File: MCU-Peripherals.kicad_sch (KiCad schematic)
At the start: 2 parts, among them J1 Conn_01x05, SW1 SW_Push

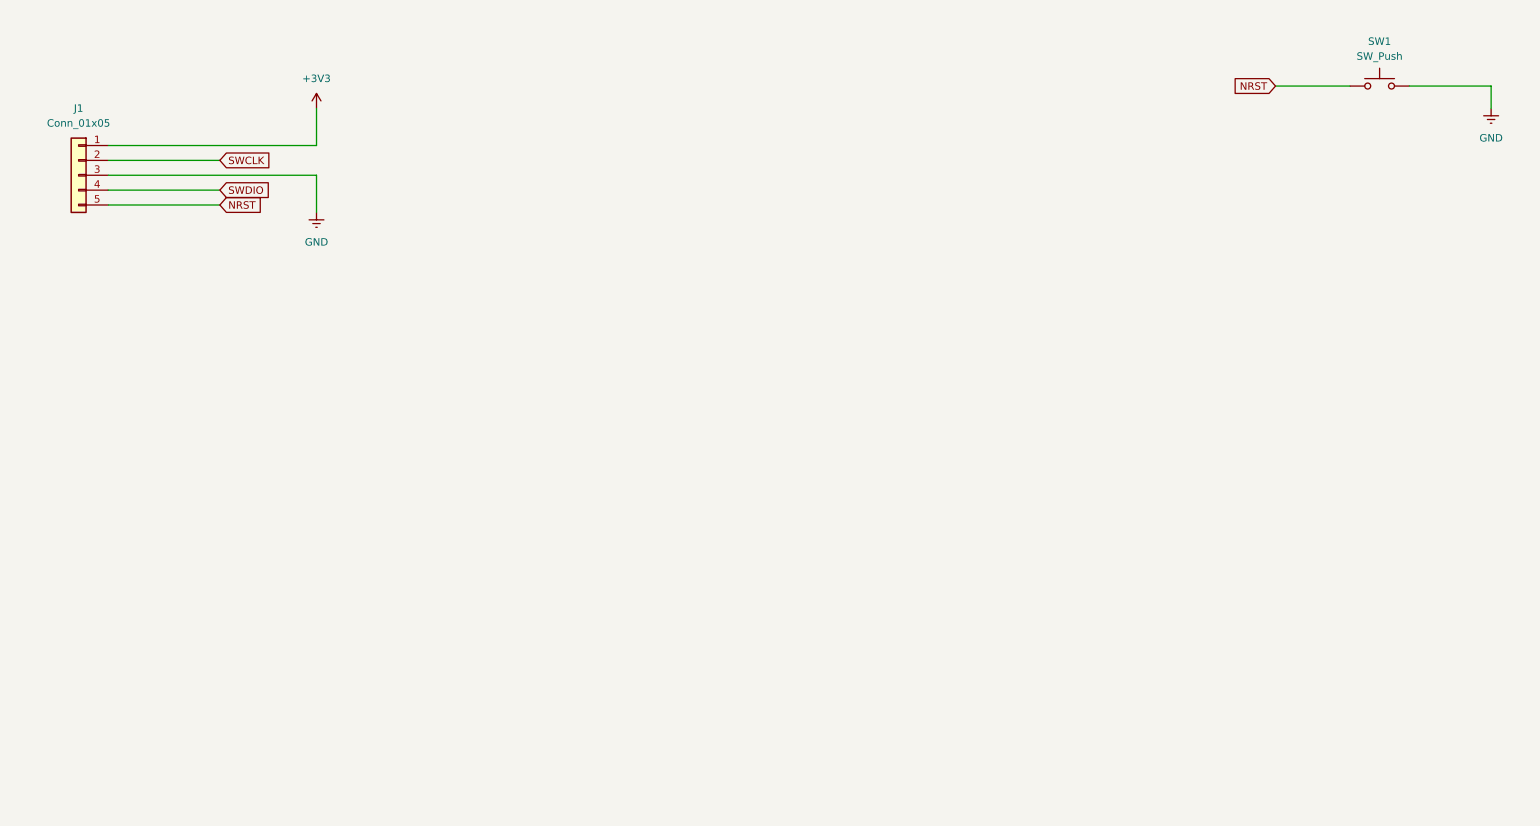
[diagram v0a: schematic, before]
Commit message: Decent progress, started USB
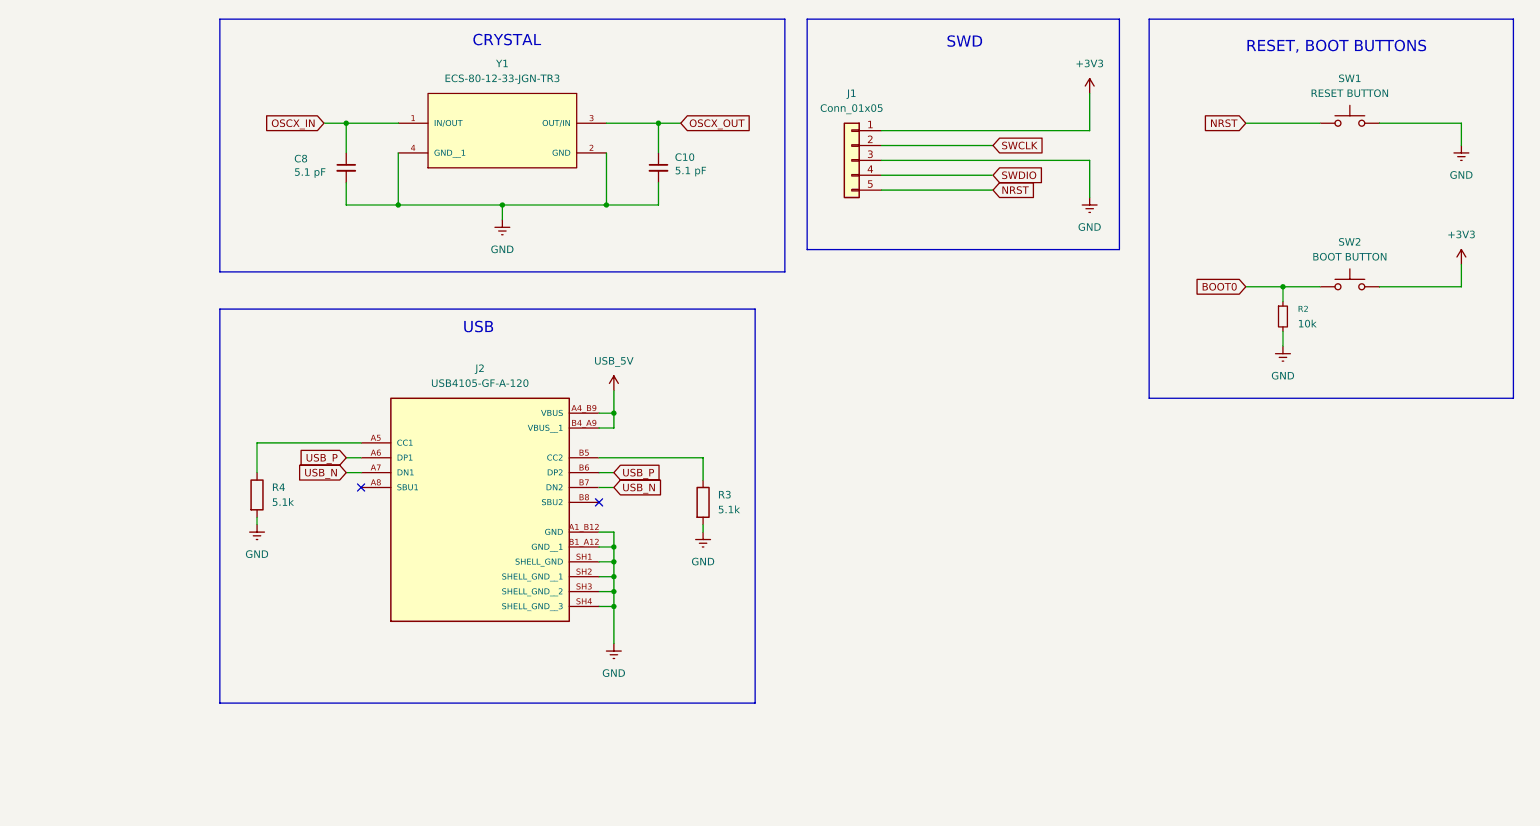
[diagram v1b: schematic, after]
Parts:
- added C10, C8: 5.1 pF, symbol Device:C_Small
- added J2: USB4105-GF-A-120, USB4105-GF-A-120:GCT_USB4105-GF-A-120, symbol USB4105-GF-A-120:USB4105-GF-A-120
- added R2: 10k, symbol Device:R_Small
- added R3, R4: 5.1k, symbol Device:R
- added SW2: BOOT BUTTON, symbol Switch:SW_Push
- added Y1: ECS-80-12-33-JGN-TR3, ECS-80-12-33-JGN-TR3:XTAL_ECS-240-8-33-AGN-TR, symbol ECS-80-12-33-JGN-TR3:ECS-80-12-33-JGN-TR3
- SW1: value SW_Push -> RESET BUTTON
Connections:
- net +3V3: now also SW2.2
- net GND: now also C10.2, C8.2, J2.A1_B12 (GND), J2.B1_A12 (GND__1), J2.SH1 (SHELL_GND), J2.SH2 (SHELL_GND__1), J2.SH3 (SHELL_GND__2), J2.SH4 (SHELL_GND__3), R2.2, R3.2, R4.2, Y1.2 (GND), Y1.4 (GND__1)
- new net: J2.A5 (CC1), R4.1
- new net: J2.B5 (CC2), R3.1
- new net BOOT0: R2.1, SW2.1
- new net OSCX_IN: C8.1, Y1.1 (IN/OUT)
- new net OSCX_OUT: C10.1, Y1.3 (OUT/IN)
- new net USB_5V: J2.A4_B9 (VBUS), J2.B4_A9 (VBUS__1)
- new net USB_N: J2.A7 (DN1), J2.B7 (DN2)
- new net USB_P: J2.A6 (DP1), J2.B6 (DP2)
- no-connect marks 0 -> 2
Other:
- note added: "CRYSTAL"
- note added: "RESET, BOOT BUTTONS"
- note added: "SWD"
- note added: "USB"
- moved on the sheet: J1, SW1

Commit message: Further schematic progress
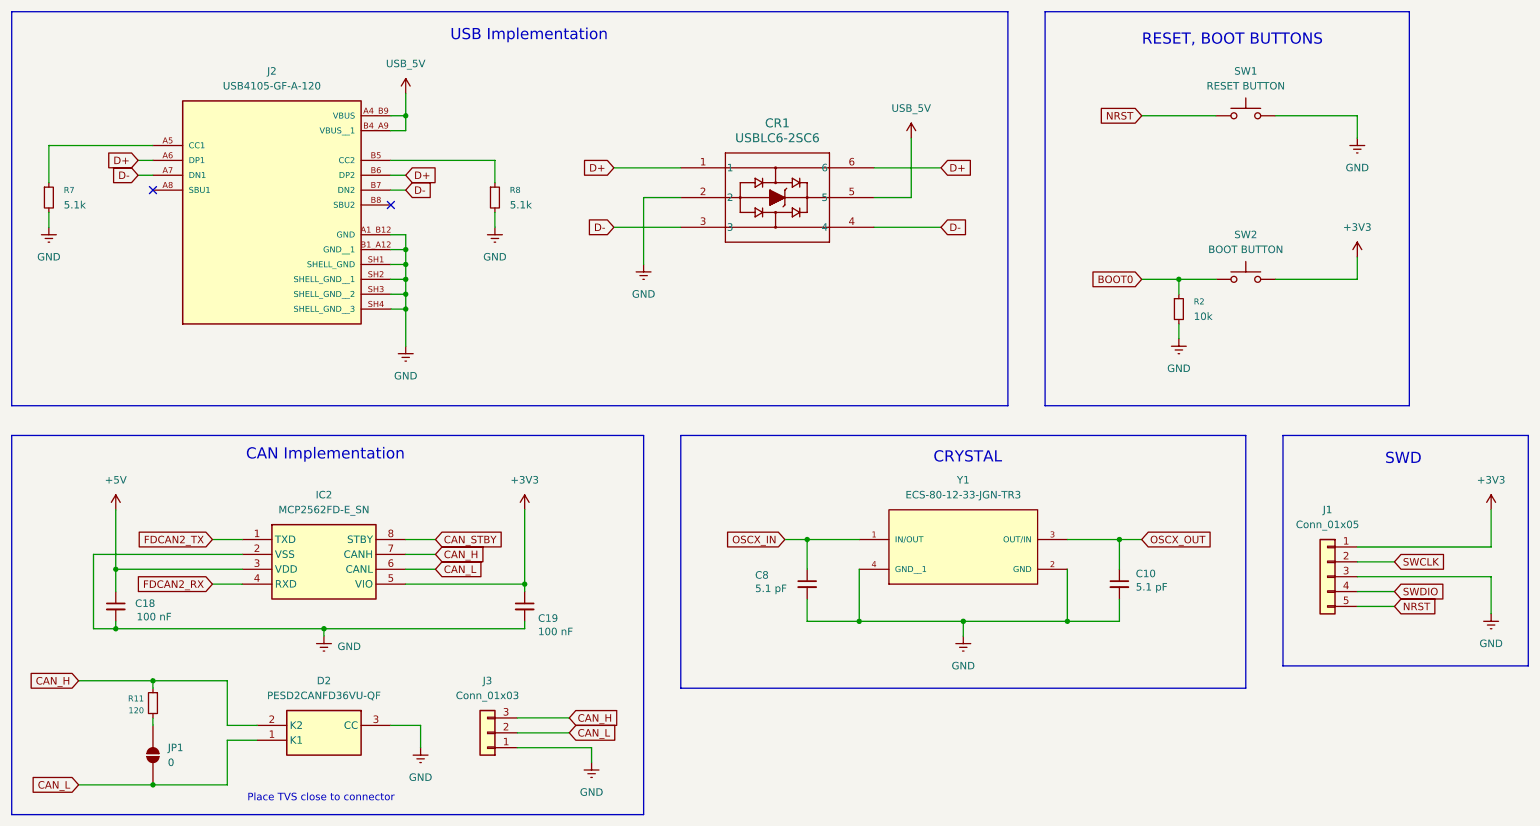
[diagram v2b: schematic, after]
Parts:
- removed R3, R4: 5.1k, symbol Device:R
- added C18, C19: 100 nF, symbol Device:C_Small
- added CR1: USBLC6-2SC6, SOT23-6L_STM, symbol USBLC6_2SC6:USBLC6-2SC6
- added D2: PESD2CANFD36VU-QF, PESD2CANFD36VUQF, symbol PESD2CANFD36VU-QF:PESD2CANFD36VU-QF
- added IC2: MCP2562FD-E_SN, SOIC127P600X175-8N, symbol MCP2562FD-E_SN:MCP2562FD-E_SN
- added J3: Conn_01x03, symbol Connector_Generic:Conn_01x03
- added JP1: 0, symbol Jumper:SolderJumper_2_Open
- added R11: 120, symbol Device:R_Small
- added R7, R8: 5.1k, symbol Device:R_Small
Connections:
- net +3V3: now also C19.1, IC2.5 (VIO)
- net GND: now also C18.2, C19.2, CR1.2, D2.3 (CC), IC2.2 (VSS), J3.1 (Pin_1), R7.2, R8.2
- net USB_5V: now also CR1.5
- net at J2.A5 (CC1): now also R7.1
- net at J2.B5 (CC2): now also R8.1
- net USB_N renamed D-
- net D-: now also CR1.3, CR1.4
- net USB_P renamed D+
- net D+: now also CR1.1, CR1.6
- new net: JP1.2 (B), R11.2
- new net +5V: C18.1, IC2.3 (VDD)
- new net CAN_H: D2.2 (K2), IC2.7 (CANH), J3.3 (Pin_3), R11.1
- new net CAN_L: D2.1 (K1), IC2.6 (CANL), J3.2 (Pin_2), JP1.1 (A)
- new net CAN_STBY: IC2.8 (STBY)
- new net FDCAN2_RX: IC2.4 (RXD)
- new net FDCAN2_TX: IC2.1 (TXD)
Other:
- note added: "CAN Implementation"
- note added: "Place TVS close to connector"
- note added: "USB Implementation"
- note removed: "USB"
- moved on the sheet: C10, C8, J1, J2, R2, SW1, SW2, Y1
